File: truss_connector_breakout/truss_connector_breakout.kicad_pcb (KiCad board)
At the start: 2 copper layers, 21 x 99.7 mm, 10 parts, among them J1 D3, J10 Truss Connector, J2 D4, J3 Servo, J4 D5, J5 D6/LC, J6 LimitSwitch, J7 D0, J8 D1, J9 D2

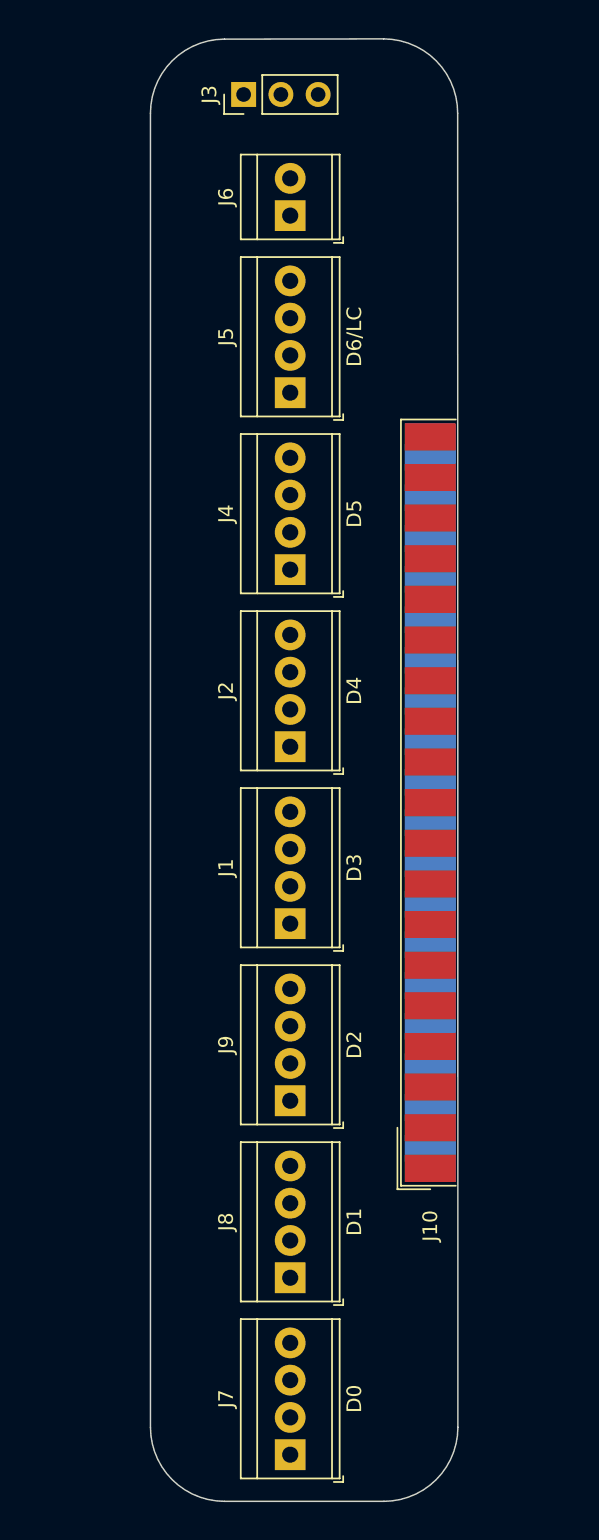
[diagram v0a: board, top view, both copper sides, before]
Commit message: update
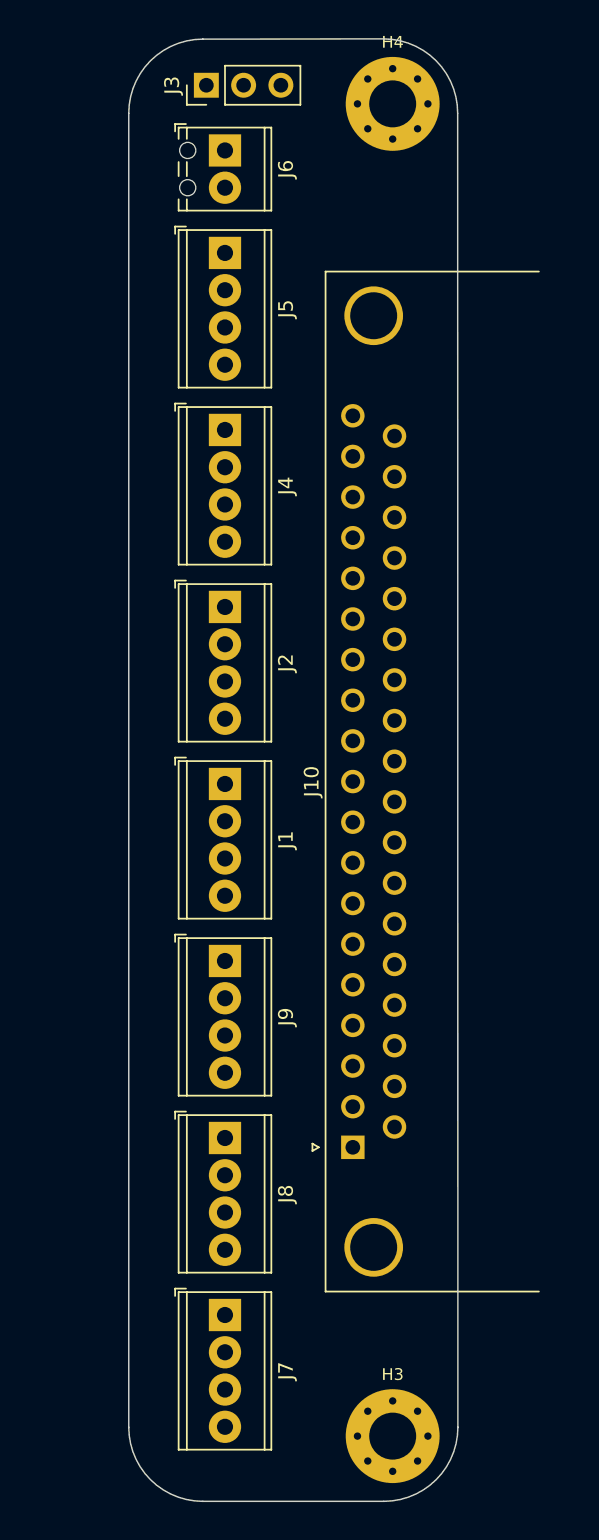
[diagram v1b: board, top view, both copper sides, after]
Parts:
- added H3: MountingHole_M3, MountingHole:MountingHole_3.2mm_M3_Pad_Via, F.Cu at (212.1, 137.2)
- added H4: MountingHole_M3, MountingHole:MountingHole_3.2mm_M3_Pad_Via, F.Cu at (212.1, 46.4)
- J1, J2, J4, J7, J8, J9: footprint TerminalBlock_TE-Connectivity:TerminalBlock_TE_282834-4_1x04_P2.54mm_Horizontal -> TerminalBlock_Phoenix:TerminalBlock_Phoenix_MPT-0,5-4-2.54_1x04_P2.54mm_Horizontal
- J10: footprint Connector_Dsub:DSUB-37_Male_EdgeMount_P2.77mm -> Connector_Dsub:DSUB-37_Male_Horizontal_P2.77x2.84mm_EdgePinOffset9.90mm_Housed_MountingHolesOffset11.32mm
- J5: value D6/LC -> D6; footprint TerminalBlock_TE-Connectivity:TerminalBlock_TE_282834-4_1x04_P2.54mm_Horizontal -> TerminalBlock_Phoenix:TerminalBlock_Phoenix_MPT-0,5-4-2.54_1x04_P2.54mm_Horizontal
- J6: footprint TerminalBlock_TE-Connectivity:TerminalBlock_TE_282834-2_1x02_P2.54mm_Horizontal -> TerminalBlock_Phoenix:TerminalBlock_Phoenix_MPT-0,5-2-2.54_1x02_P2.54mm_Horizontal
- moved J10 24.1 mm to (209.4, 117.5)
- moved J2 10.5 mm to (200.7, 80.6), turned to -90 degrees
- moved J5 10.5 mm to (200.7, 56.5), turned to -90 degrees
- moved J8 10.5 mm to (200.7, 116.8), turned to -90 degrees
- moved J9 10.5 mm to (200.7, 104.8), turned to -90 degrees
- moved J1 10.5 mm to (200.7, 92.7), turned to -90 degrees
- moved J7 10.5 mm to (200.7, 128.9), turned to -90 degrees
- moved J4 10.5 mm to (200.7, 68.6), turned to -90 degrees
- moved J6 6.28 mm to (200.7, 49.5), turned to -90 degrees
- moved J3 2.62 mm to (199.4, 45.1)
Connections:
- J1 pad 1: /D3_VCC -> /D3_LC+
- J1 pad 2: /D3_GND -> /D3_LC-
- J1 pad 3: /D3_LC- -> /D3_GND
- J1 pad 4: /D3_LC+ -> /D3_VCC
- J2 pad 1: /D4_VCC -> /D4_LC+
- J2 pad 2: /D4_GND -> /D4_LC-
- J2 pad 3: /D4_LC- -> /D4_GND
- J2 pad 4: /D4_LC+ -> /D4_VCC
- J4 pad 1: /D5_VCC -> /D5_LC+
- J4 pad 2: /D5_GND -> /D5_LC-
- J4 pad 3: /D5_LC- -> /D5_GND
- J4 pad 4: /D5_LC+ -> /D5_VCC
- J5 pad 1: /D6_VCC -> /D6_LC+
- J5 pad 2: /D6_GND -> /D6_LC-
- J5 pad 3: /D6_LC- -> /D6_GND
- J5 pad 4: /D6_LC+ -> /D6_VCC
- J6 pad 1: /LIMIT_SWITCH -> /LS_GND
- J6 pad 2: /LS_GND -> /LIMIT_SWITCH
- J7 pad 1: /D0_VCC -> /D0_LC+
- J7 pad 2: /D0_GND -> /D0_LC-
- J7 pad 3: /D0_LC- -> /D0_GND
- J7 pad 4: /D0_LC+ -> /D0_VCC
- J8 pad 1: /D1_VCC -> /D1_LC+
- J8 pad 2: /D1_GND -> /D1_LC-
- J8 pad 3: /D1_LC- -> /D1_GND
- J8 pad 4: /D1_LC+ -> /D1_VCC
- J9 pad 1: /D2_VCC -> /D2_LC+
- J9 pad 2: /D2_GND -> /D2_LC-
- J9 pad 3: /D2_LC- -> /D2_GND
- J9 pad 4: /D2_LC+ -> /D2_VCC
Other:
- board size 21 x 99.7 mm -> 22.4 x 99.7 mm

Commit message: updating truss PCB
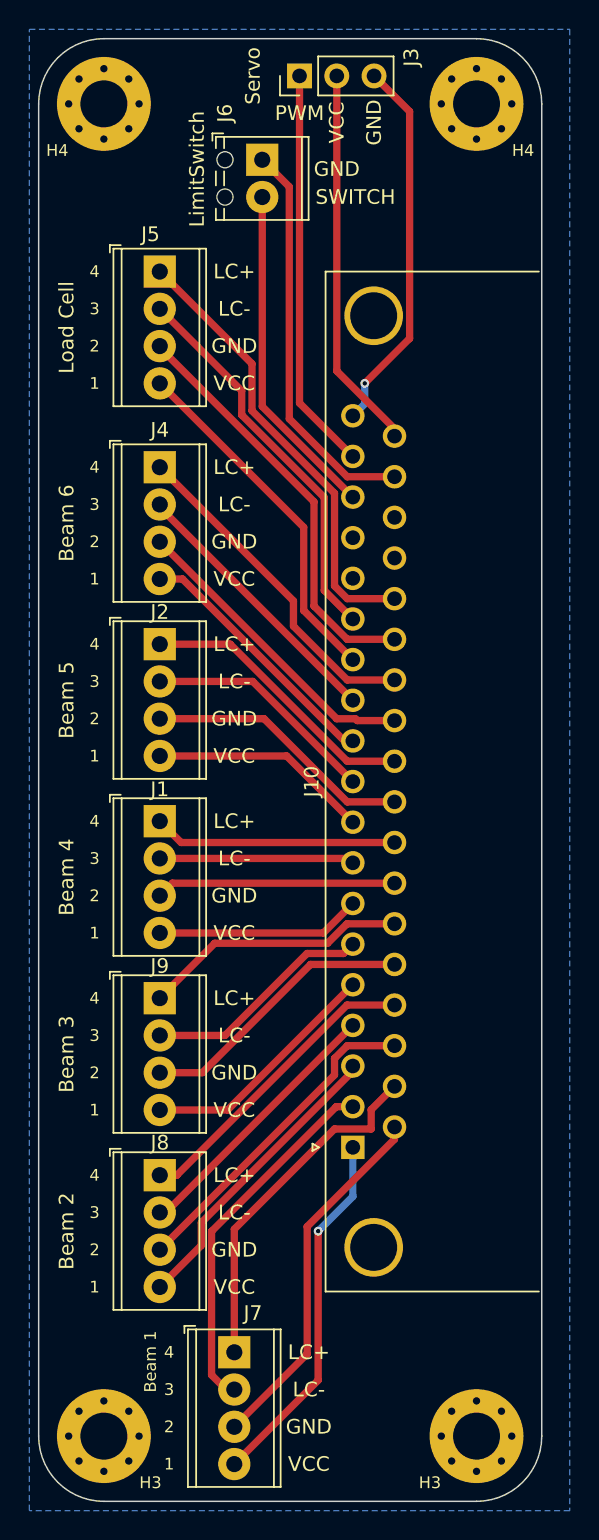
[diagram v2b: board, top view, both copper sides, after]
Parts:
- added H3: MountingHole_M3, MountingHole:MountingHole_3.2mm_M3_Pad_Via, F.Cu at (192.4, 137.2)
- added H4: MountingHole_M3, MountingHole:MountingHole_3.2mm_M3_Pad_Via, F.Cu at (192.4, 46.4)
- moved J3 6.38 mm to (205.7, 44.5)
- moved H3 5.72 mm to (217.8, 137.2)
- moved H4 5.72 mm to (217.8, 46.4)
- moved J4 5.12 mm to (196.2, 71.1)
- moved J1 5.12 mm to (196.2, 95.2)
- moved J2 5.12 mm to (196.2, 83.2)
- moved J8 5.12 mm to (196.2, 119.4)
- moved J9 5.12 mm to (196.2, 107.3)
- moved J5 4.62 mm to (196.2, 57.8)
- moved J6 2.62 mm to (203.2, 50.2)
- moved J7 2.62 mm to (201.3, 131.4)
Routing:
- net /D6_LC+: track 0.00 -> 30.8 mm
- net /D6_GND: track 0.00 -> 28.5 mm
- net /PWM_SERVO: track 0.00 -> 27.4 mm
- net /LS_GND: track 0.00 -> 27.2 mm
- net /D6_LC-: track 0.00 -> 26.6 mm
- net /SERVO_VCC: track 0.00 -> 26.2 mm
- net /SERVO_GND: track 0.00 -> 25.8 mm, vias 0 -> 1
- net /D0_GND: track 0.00 -> 25.0 mm
- net /D0_VCC: track 0.00 -> 24.9 mm, vias 0 -> 1
- net /D0_LC-: track 0.00 -> 24.9 mm
- net /D6_VCC: track 0.00 -> 24.3 mm
- net /D0_LC+: track 0.00 -> 24.1 mm
- net /D5_LC+: track 0.00 -> 23.0 mm
- net /LIMIT_SWITCH: track 0.00 -> 23.0 mm
- net /D1_GND: track 0.00 -> 22.4 mm
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- added copper zone on B.Cu, net GND
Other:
- board size 22.4 x 99.7 mm -> 34.3 x 99.7 mm
- board text added: "1"
- board text added: "2"
- board text added: "3"
- board text added: "4"
- board text added: "Beam 1"
- board text added: "Beam 2"
- board text added: "Beam 3"
- board text added: "Beam 4"
- board text added: "Beam 5"
- board text added: "Beam 6"
- board text added: "GND"
- board text added: "LC+"
- board text added: "LC-"
- board text added: "Load Cell"
- board text added: "PWM"
- board text added: "SWITCH"
- board text added: "VCC"
